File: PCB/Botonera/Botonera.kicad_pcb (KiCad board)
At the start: 2 copper layers, 42.4 x 57.2 mm, 9 parts, among them P1 DIN_5

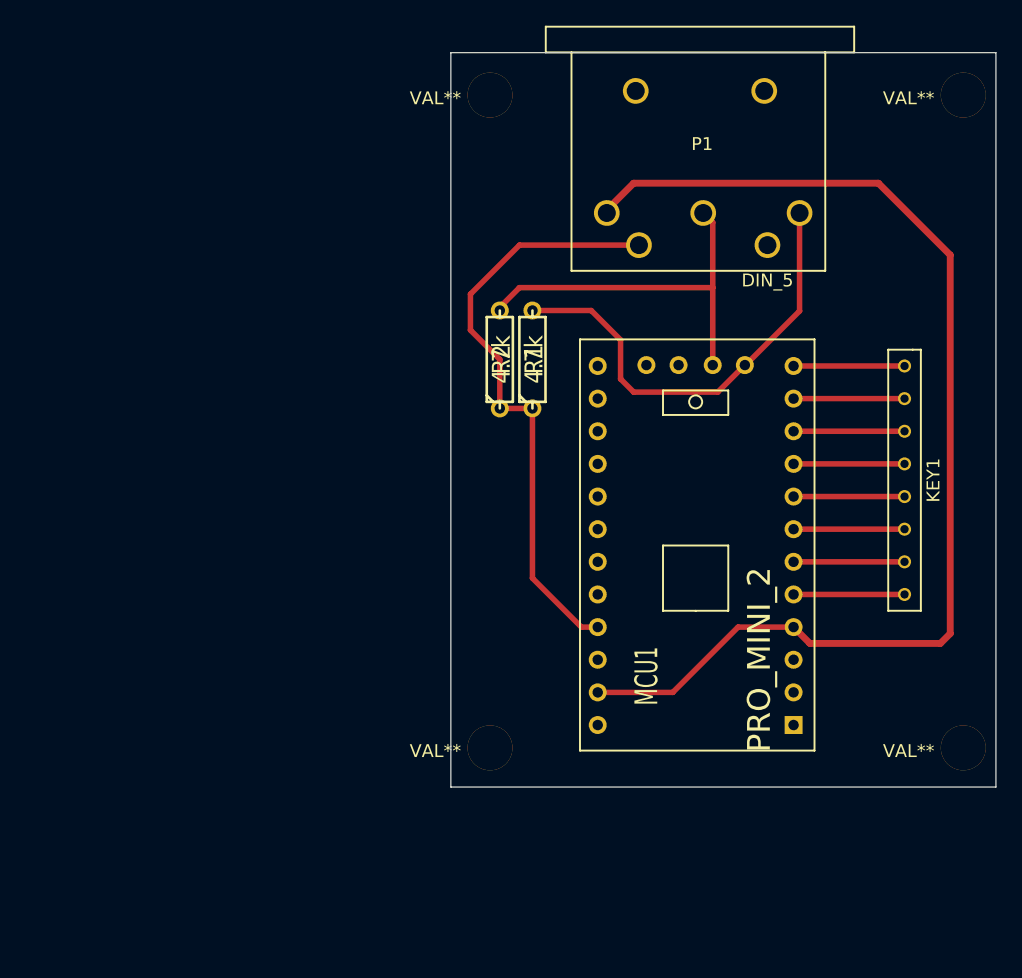
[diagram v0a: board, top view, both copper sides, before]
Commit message: Botonera
Botonera
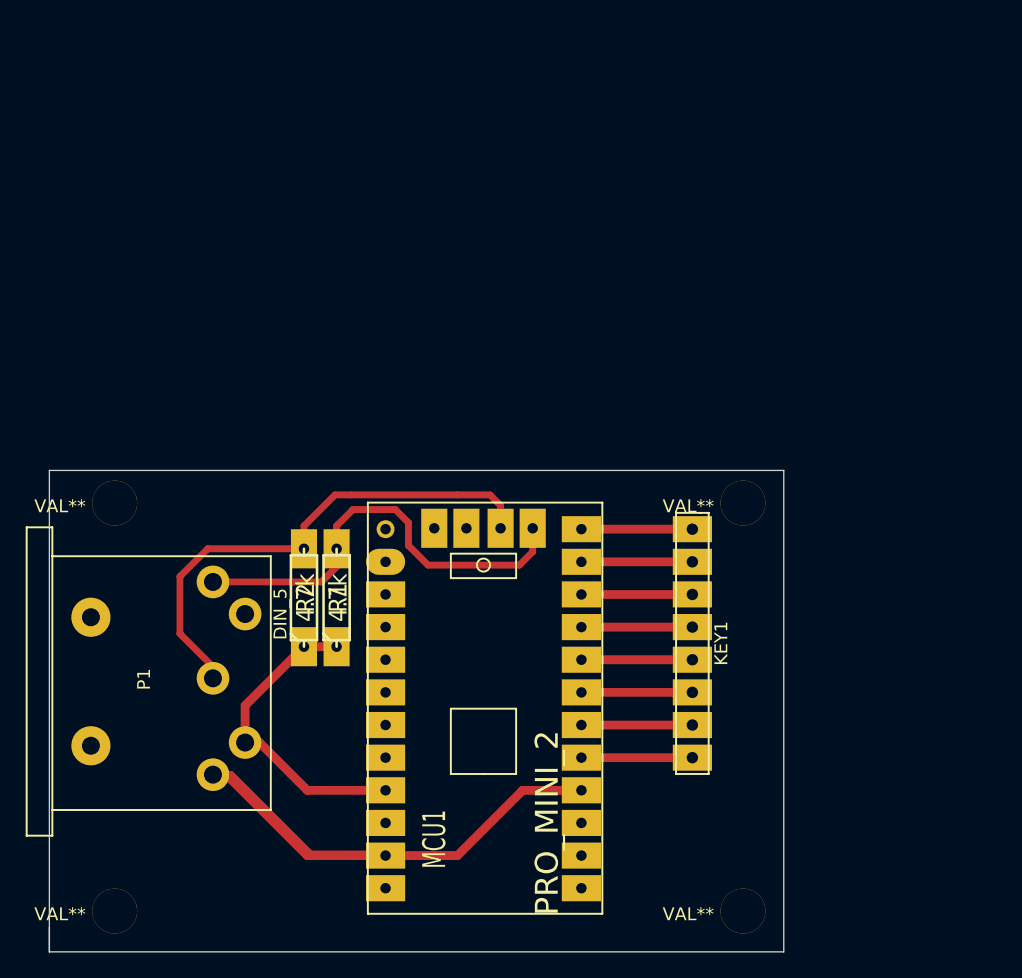
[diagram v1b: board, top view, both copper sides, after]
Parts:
- moved P1 50.5 mm to (75.7, 69.6), turned to 270 degrees
- moved 3.5mm_Screw 43.1 mm to (66.0, 61.0)
- moved 3.5mm_Screw 36.1 mm to (114.9, 61.0)
- moved 3.5mm_Screw 31.9 mm to (66.0, 92.7)
- moved R1 24.0 mm to (83.3, 68.3)
- moved R2 24.0 mm to (80.8, 68.3)
- moved 3.5mm_Screw 21.3 mm to (114.9, 92.7)
- moved KEY1 20.8 mm to (111.0, 71.9)
- moved MCU1 20.8 mm to (94.7, 74.4)
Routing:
- net GND: track 90.0 -> 50.1 mm
- net +5V: track 46.9 -> 30.8 mm
- net I2CSDA: track 29.6 -> 39.7 mm
- net I2CSCL: track 35.4 -> 34.2 mm
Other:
- board size 42.4 x 57.2 mm -> 57.1 x 37.5 mm

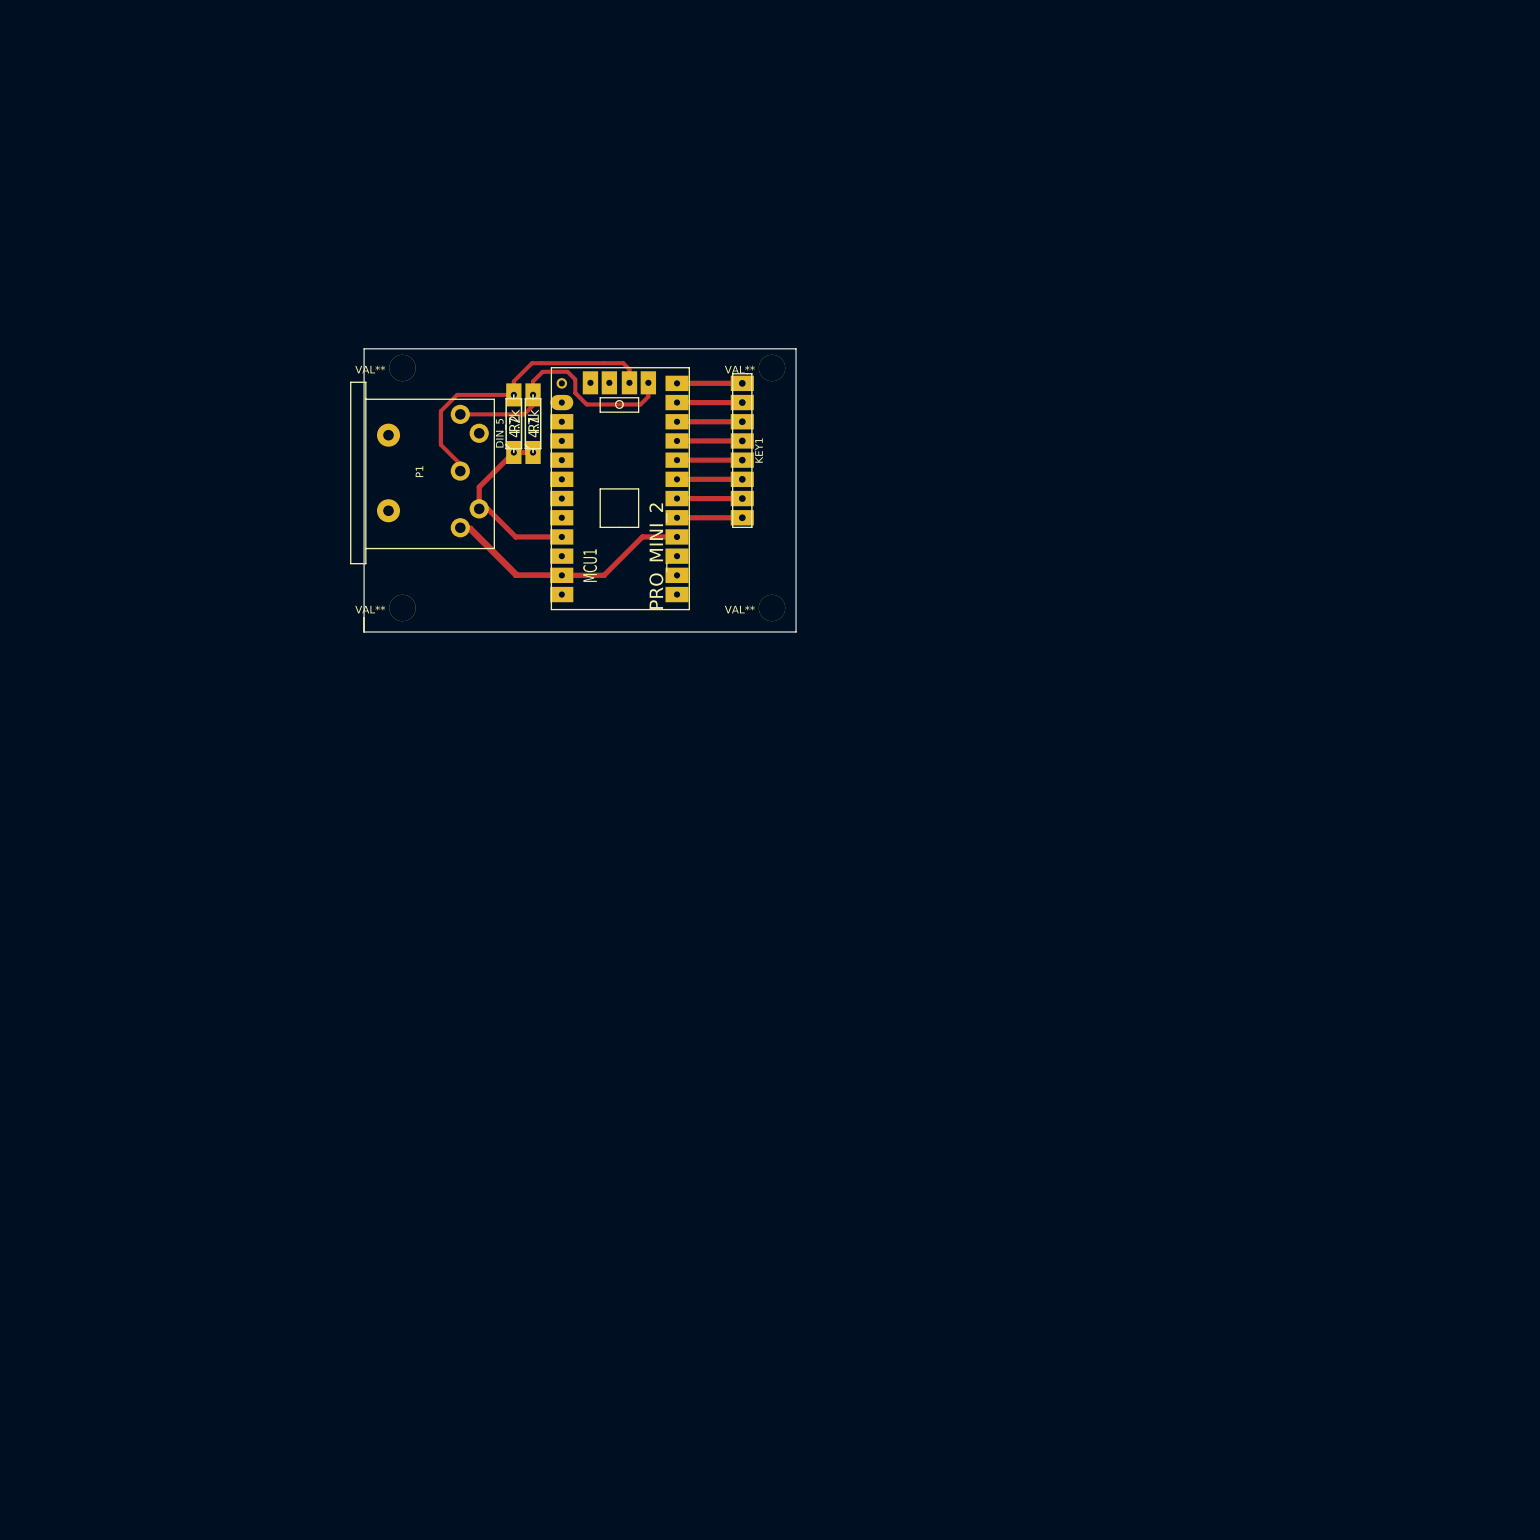
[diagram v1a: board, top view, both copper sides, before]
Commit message: Botonera Panel
Botonera Panel
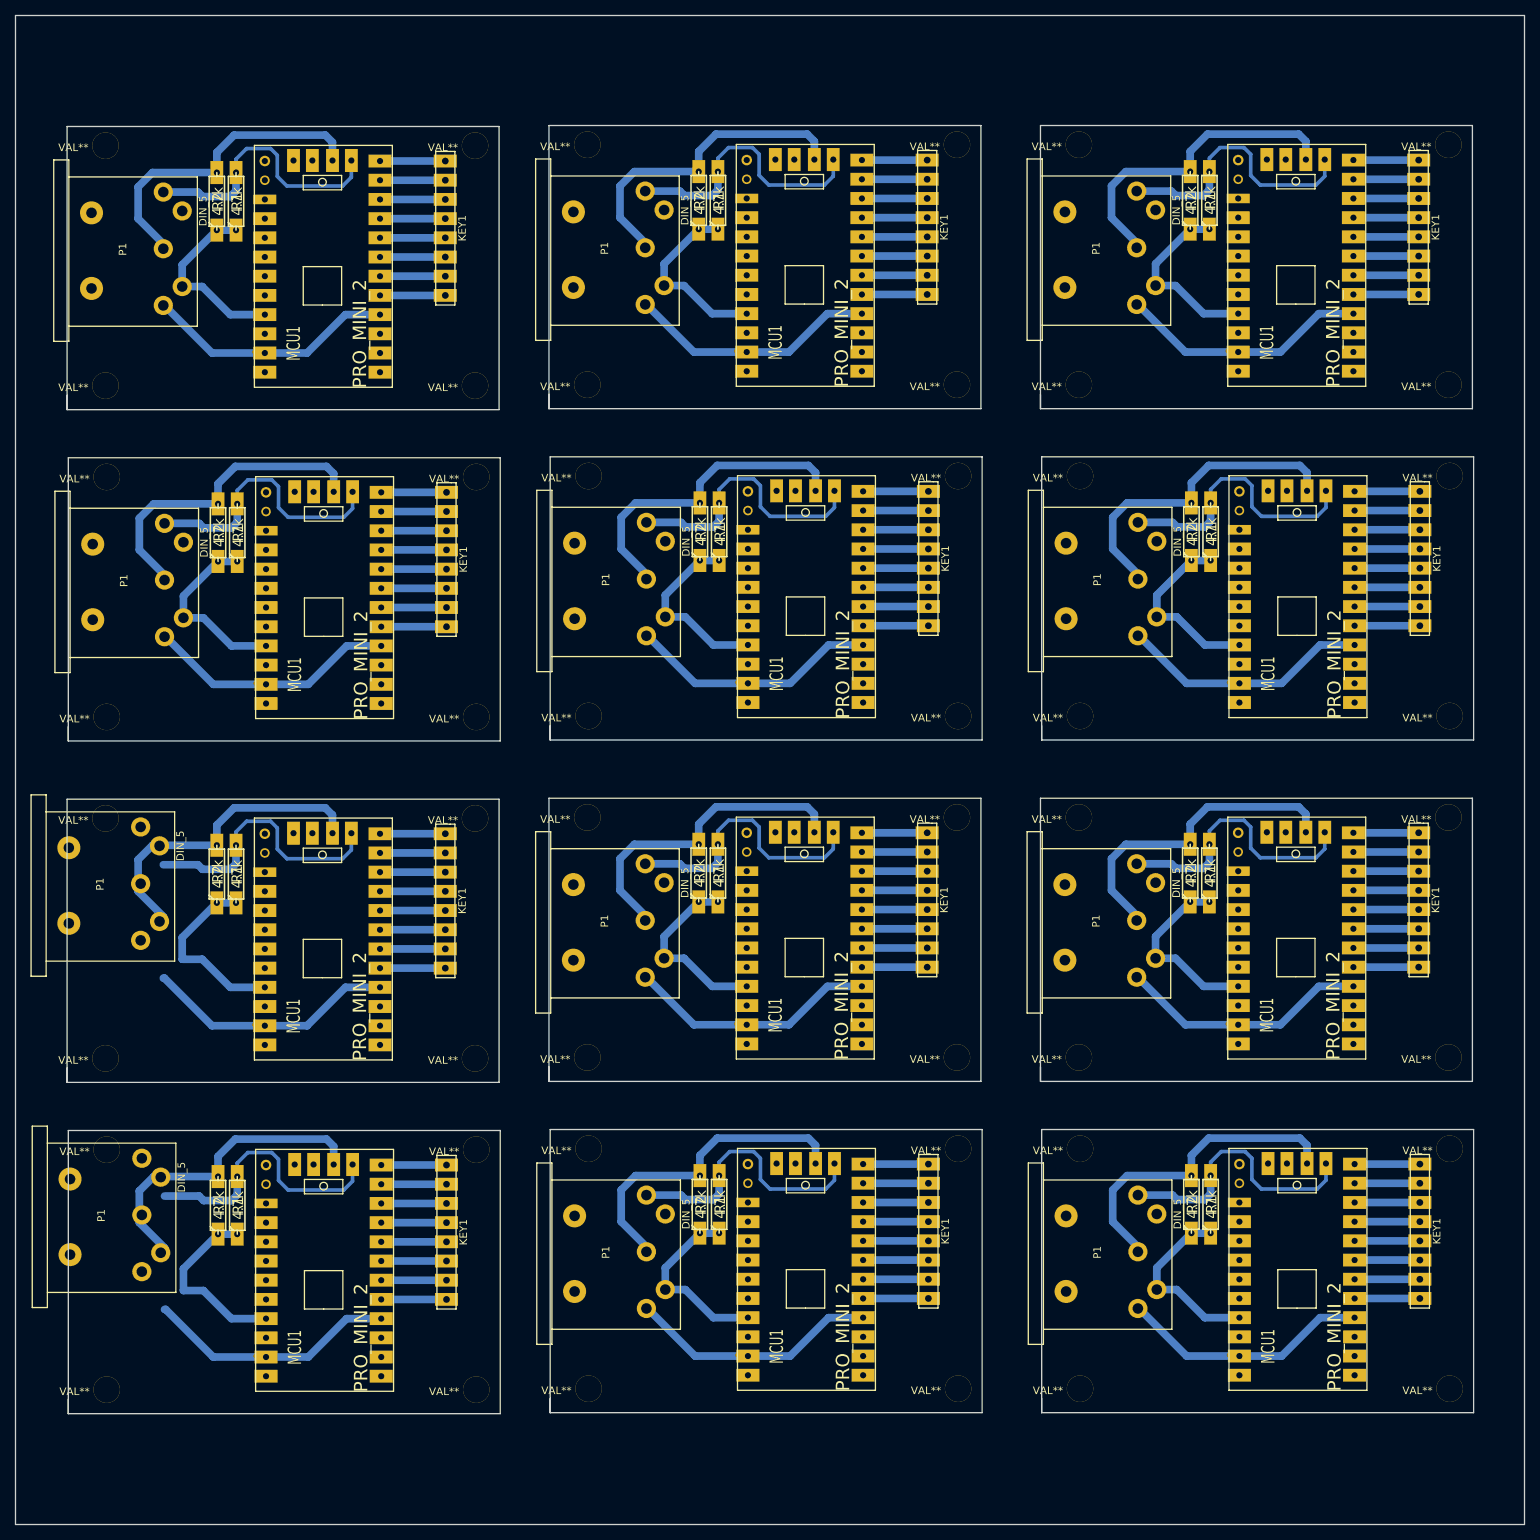
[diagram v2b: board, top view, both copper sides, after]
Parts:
- removed the MCU1 at (94.7, 74.4)
- removed the P1 at (75.7, 69.6)
- added 3.5mm_Screw: VAL**, 3.5mm_Screw, F.Cu at (90.5, 152.2)
- added 3.5mm_Screw: VAL**, 3.5mm_Screw, F.Cu at (204.4, 120.4)
- added 3.5mm_Screw: VAL**, 3.5mm_Screw, F.Cu at (204.4, 152.2)
- added 3.5mm_Screw: VAL**, 3.5mm_Screw, F.Cu at (155.5, 152.2)
- added 3.5mm_Screw: VAL**, 3.5mm_Screw, F.Cu at (155.7, 196.0)
- added 3.5mm_Screw: VAL**, 3.5mm_Screw, F.Cu at (204.6, 196.0)
- added 3.5mm_Screw: VAL**, 3.5mm_Screw, F.Cu at (204.6, 164.2)
- added 3.5mm_Screw: VAL**, 3.5mm_Screw, F.Cu at (155.7, 164.2)
- added 3.5mm_Screw: VAL**, 3.5mm_Screw, F.Cu at (26.9, 196.1)
- added 3.5mm_Screw: VAL**, 3.5mm_Screw, F.Cu at (75.8, 196.1)
- added 3.5mm_Screw: VAL**, 3.5mm_Screw, F.Cu at (75.8, 164.4)
- added 3.5mm_Screw: VAL**, 3.5mm_Screw, F.Cu at (139.4, 152.2)
- added 3.5mm_Screw: VAL**, 3.5mm_Screw, F.Cu at (26.9, 164.4)
- added 3.5mm_Screw: VAL**, 3.5mm_Screw, F.Cu at (90.7, 164.2)
- added 3.5mm_Screw: VAL**, 3.5mm_Screw, F.Cu at (139.6, 164.2)
- added 3.5mm_Screw: VAL**, 3.5mm_Screw, F.Cu at (139.6, 196.0)
- added 3.5mm_Screw: VAL**, 3.5mm_Screw, F.Cu at (90.7, 196.0)
- added 3.5mm_Screw: VAL**, 3.5mm_Screw, F.Cu at (90.7, 107.0)
- added 3.5mm_Screw: VAL**, 3.5mm_Screw, F.Cu at (139.6, 107.0)
- added 3.5mm_Screw: VAL**, 3.5mm_Screw, F.Cu at (139.6, 75.2)
- added 3.5mm_Screw: VAL**, 3.5mm_Screw, F.Cu at (90.7, 75.2)
- added 3.5mm_Screw: VAL**, 3.5mm_Screw, F.Cu at (26.9, 75.4)
- added 3.5mm_Screw: VAL**, 3.5mm_Screw, F.Cu at (139.4, 120.4)
- added 3.5mm_Screw: VAL**, 3.5mm_Screw, F.Cu at (75.8, 75.4)
- added 3.5mm_Screw: VAL**, 3.5mm_Screw, F.Cu at (75.8, 107.1)
- added 3.5mm_Screw: VAL**, 3.5mm_Screw, F.Cu at (26.9, 107.1)
- added 3.5mm_Screw: VAL**, 3.5mm_Screw, F.Cu at (155.7, 75.2)
- added 3.5mm_Screw: VAL**, 3.5mm_Screw, F.Cu at (204.6, 75.2)
- added 3.5mm_Screw: VAL**, 3.5mm_Screw, F.Cu at (204.6, 107.0)
- added 3.5mm_Screw: VAL**, 3.5mm_Screw, F.Cu at (155.7, 107.0)
- added 3.5mm_Screw: VAL**, 3.5mm_Screw, F.Cu at (155.5, 63.2)
- added 3.5mm_Screw: VAL**, 3.5mm_Screw, F.Cu at (204.4, 63.2)
- added 3.5mm_Screw: VAL**, 3.5mm_Screw, F.Cu at (204.4, 31.4)
- added 3.5mm_Screw: VAL**, 3.5mm_Screw, F.Cu at (90.5, 120.4)
- added 3.5mm_Screw: VAL**, 3.5mm_Screw, F.Cu at (155.5, 31.4)
- added 3.5mm_Screw: VAL**, 3.5mm_Screw, F.Cu at (26.7, 63.3)
- added 3.5mm_Screw: VAL**, 3.5mm_Screw, F.Cu at (75.6, 63.3)
- added 3.5mm_Screw: VAL**, 3.5mm_Screw, F.Cu at (75.6, 31.5)
- added 3.5mm_Screw: VAL**, 3.5mm_Screw, F.Cu at (26.7, 31.5)
- added 3.5mm_Screw: VAL**, 3.5mm_Screw, F.Cu at (26.7, 120.5)
- added 3.5mm_Screw: VAL**, 3.5mm_Screw, F.Cu at (75.6, 120.5)
- added 3.5mm_Screw: VAL**, 3.5mm_Screw, F.Cu at (75.6, 152.3)
- added 3.5mm_Screw: VAL**, 3.5mm_Screw, F.Cu at (26.7, 152.3)
- added 3.5mm_Screw: VAL**, 3.5mm_Screw, F.Cu at (155.5, 120.4)
- added KEY1: KEYPAD_4X4, PinArray_8x1, F.Cu at (135.5, 131.3)
- added KEY1: KEYPAD_4X4, PinArray_8x1, F.Cu at (200.5, 42.3)
- added KEY1: KEYPAD_4X4, PinArray_8x1, F.Cu at (71.7, 42.5)
- added KEY1: KEYPAD_4X4, PinArray_8x1, F.Cu at (71.7, 131.5)
- added KEY1: KEYPAD_4X4, PinArray_8x1, F.Cu at (200.5, 131.3)
- added KEY1: KEYPAD_4X4, PinArray_8x1, F.Cu at (200.6, 175.2)
- added KEY1: KEYPAD_4X4, PinArray_8x1, F.Cu at (71.9, 175.3)
- added KEY1: KEYPAD_4X4, PinArray_8x1, F.Cu at (135.6, 175.2)
- added KEY1: KEYPAD_4X4, PinArray_8x1, F.Cu at (135.6, 86.2)
- added KEY1: KEYPAD_4X4, PinArray_8x1, F.Cu at (71.9, 86.3)
- added KEY1: KEYPAD_4X4, PinArray_8x1, F.Cu at (200.6, 86.2)
- added MCU1: PRO_MINI_2, ProMini2, F.Cu at (119.2, 133.9)
- added MCU1: PRO_MINI_2, ProMini2, F.Cu at (184.2, 44.9)
- added MCU1: PRO_MINI_2, ProMini2, F.Cu at (55.5, 45.0)
- added MCU1: PRO_MINI_2, ProMini2, F.Cu at (119.2, 44.9)
- added MCU1: PRO_MINI_2, ProMini2, F.Cu at (55.5, 134.0)
- added MCU1: PRO_MINI_2, ProMini2, F.Cu at (184.2, 133.9)
- added MCU1: PRO_MINI_2, ProMini2, F.Cu at (184.4, 177.7)
- added MCU1: PRO_MINI_2, ProMini2, F.Cu at (55.6, 177.8)
- added MCU1: PRO_MINI_2, ProMini2, F.Cu at (119.4, 177.7)
- added MCU1: PRO_MINI_2, ProMini2, F.Cu at (119.4, 88.7)
- added MCU1: PRO_MINI_2, ProMini2, F.Cu at (55.6, 88.8)
- added MCU1: PRO_MINI_2, ProMini2, F.Cu at (184.4, 88.7)
- added P1: DIN_5, DIN5, F.Cu at (100.2, 129.1)
- added P1: DIN_5, DIN5, F.Cu at (165.2, 40.1)
- added P1: DIN_5, DIN5, F.Cu at (36.4, 40.2)
- added P1: DIN_5, DIN5, F.Cu at (100.2, 40.1)
- added P1: DIN_5, DIN5, F.Cu at (33.4, 124.2)
- added P1: DIN_5, DIN5, F.Cu at (165.2, 129.1)
- added P1: DIN_5, DIN5, F.Cu at (165.3, 172.9)
- added P1: DIN_5, DIN5, F.Cu at (33.6, 168.0)
- added P1: DIN_5, DIN5, F.Cu at (100.3, 172.9)
- added P1: DIN_5, DIN5, F.Cu at (100.3, 83.9)
- added P1: DIN_5, DIN5, F.Cu at (36.6, 84.0)
- added P1: DIN_5, DIN5, F.Cu at (165.3, 83.9)
- added R1: 4.7k, R3, F.Cu at (107.8, 127.8)
- added R1: 4.7k, R3, F.Cu at (172.8, 38.8)
- added R1: 4.7k, R3, F.Cu at (44.0, 38.9)
- added R1: 4.7k, R3, F.Cu at (44.0, 127.9)
- added R1: 4.7k, R3, F.Cu at (172.8, 127.8)
- added R1: 4.7k, R3, F.Cu at (173.0, 171.6)
- added R1: 4.7k, R3, F.Cu at (44.2, 171.7)
- added R1: 4.7k, R3, F.Cu at (107.9, 171.6)
- added R1: 4.7k, R3, F.Cu at (107.9, 82.6)
- added R1: 4.7k, R3, F.Cu at (44.2, 82.7)
- added R1: 4.7k, R3, F.Cu at (173.0, 82.6)
- added R2: 4.7k, R3, F.Cu at (105.2, 127.8)
- added R2: 4.7k, R3, F.Cu at (170.3, 38.8)
- added R2: 4.7k, R3, F.Cu at (41.5, 38.9)
- added R2: 4.7k, R3, F.Cu at (41.5, 127.9)
- added R2: 4.7k, R3, F.Cu at (170.3, 127.8)
- added R2: 4.7k, R3, F.Cu at (170.4, 171.6)
- added R2: 4.7k, R3, F.Cu at (41.6, 171.7)
- added R2: 4.7k, R3, F.Cu at (105.4, 171.6)
- added R2: 4.7k, R3, F.Cu at (105.4, 82.6)
- added R2: 4.7k, R3, F.Cu at (41.6, 82.7)
- added R2: 4.7k, R3, F.Cu at (170.4, 82.6)
- moved KEY1 38.4 mm to (135.5, 42.3)
- moved 3.5mm_Screw 38.4 mm to (90.5, 31.4)
- moved 3.5mm_Screw 38.4 mm to (139.4, 31.4)
- moved 3.5mm_Screw 38.4 mm to (139.4, 63.2)
- moved 3.5mm_Screw 38.4 mm to (90.5, 63.2)
- moved R1 38.4 mm to (107.8, 38.8)
- moved R2 38.4 mm to (105.2, 38.8)
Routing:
- net I2CSDA: track 39.7 -> 508.4 mm
- net I2CSCL: track 34.2 -> 439.1 mm
- net GND: track 50.1 -> 425.6 mm
- net +5V: track 30.8 -> 293.7 mm
- net N-000009: track 8.64 -> 103.6 mm
- net N-000004: track 8.64 -> 103.6 mm
- net N-000003: track 8.64 -> 103.6 mm
- net N-0000027: track 8.64 -> 103.6 mm
- net N-0000026: track 8.64 -> 103.6 mm
- net N-0000025: track 8.64 -> 103.6 mm
- net N-0000024: track 8.64 -> 103.6 mm
- net N-000002: track 8.64 -> 103.6 mm
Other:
- board size 57.1 x 37.5 mm -> 199.6 x 199.6 mm
- net class Default: clearance 0.254 -> 0.635
- rule trace_clearance: 0.254 -> 0.635
